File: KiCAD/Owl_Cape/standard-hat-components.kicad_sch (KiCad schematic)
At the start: 12 parts, among them Q1 MMDT5401, Q2 DMG2302U, U1 AT24C256C

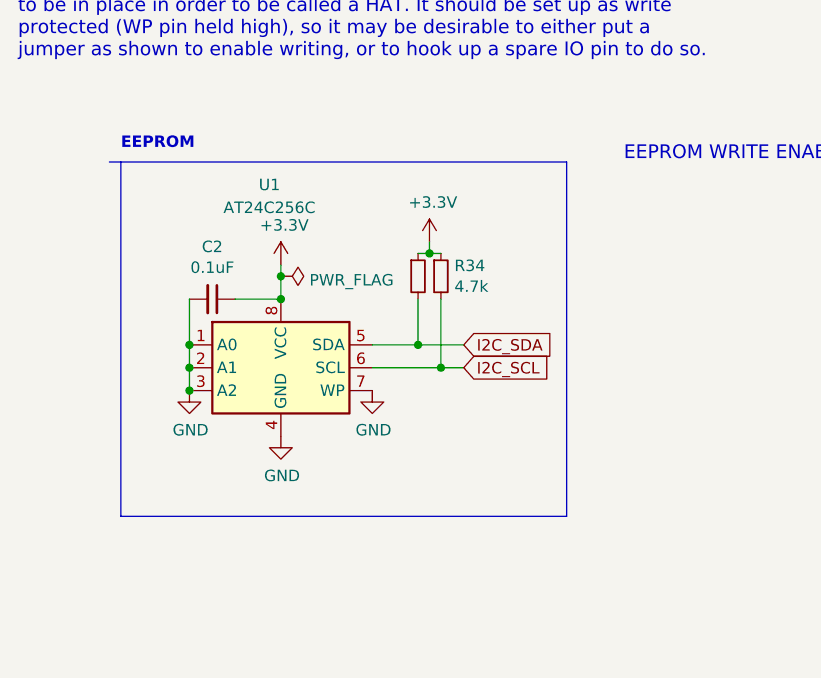
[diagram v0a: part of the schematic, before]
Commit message: formatting fix
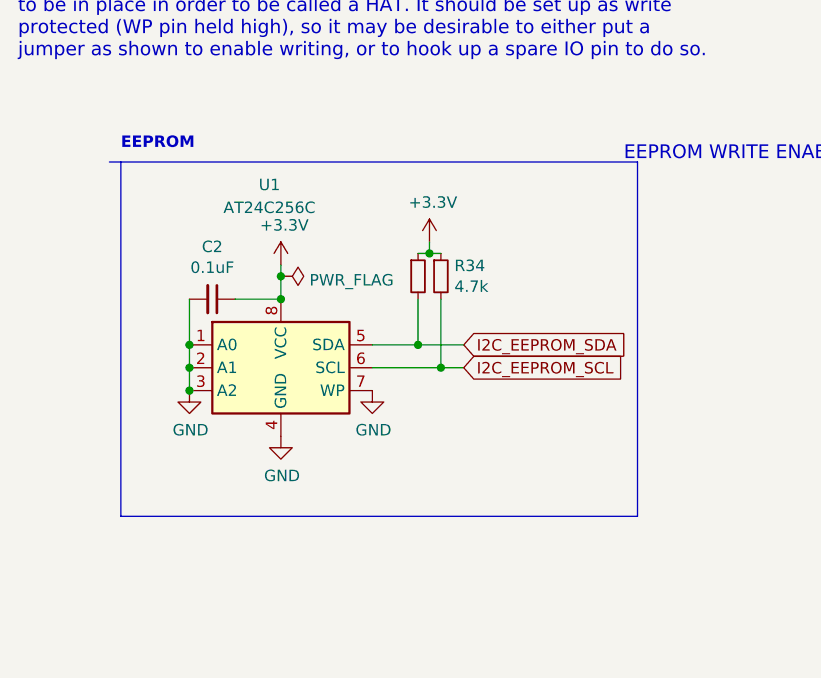
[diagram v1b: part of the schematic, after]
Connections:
- net I2C_SCL renamed I2C_EEPROM_SCL
- net I2C_SDA renamed I2C_EEPROM_SDA
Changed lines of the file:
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@@
     (stroke (width 0) (type default) (color 0 0 0 0))
   )
-  (polyline (pts (xy 80.01 62.23) (xy 80.01 101.6))
+  (polyline (pts (xy 87.884 62.23) (xy 87.884 101.6))
     (stroke (width 0) (type default) (color 0 0 0 0))
   )
@@
     (stroke (width 0) (type default) (color 0 0 0 0))
   )
-  (polyline (pts (xy 80.01 101.6) (xy 30.48 101.6))
+  (polyline (pts (xy 87.884 101.6) (xy 30.48 101.6))
     (stroke (width 0) (type default) (color 0 0 0 0))
   )
@@
     (stroke (width 0) (type default) (color 0 0 0 0))
   )
-  (polyline (pts (xy 29.21 62.23) (xy 80.01 62.23))
+  (polyline (pts (xy 29.21 62.23) (xy 87.884 62.23))
     (stroke (width 0) (type default) (color 0 0 0 0))
   )
@@
     (effects (font (size 1.524 1.524)) (justify left bottom))
   )
-  (global_label "I2C_SCL" (shape input) (at 68.58 85.09 0) (fields_autoplaced)
+  (global_label "I2C_EEPROM_SCL" (shape input) (at 68.58 85.09 0) (fields_autoplaced)
     (effects (font (size 1.27 1.27)) (justify left))
-    (property "Intersheet References" "${INTERSHEET_REFS}" (id 0) (at 3.81 8.89 0)
-      (effects (font (size 1.27 1.27)) hide)
+    (property "Intersheet References" "${INTERSHEET_REFS}" (id 0) (at 87.0513 85.0106 0)
+      (effects (font (size 1.27 1.27)) (justify left) hide)
     )
   )
-  (global_label "I2C_SDA" (shape input) (at 68.58 82.55 0) (fields_autoplaced)
+  (global_label "I2C_EEPROM_SDA" (shape input) (at 68.58 82.55 0) (fields_autoplaced)
     (effects (font (size 1.27 1.27)) (justify left))
-    (property "Intersheet References" "${INTERSHEET_REFS}" (id 0) (at 3.81 8.89 0)
-      (effects (font (size 1.27 1.27)) hide)
+    (property "Intersheet References" "${INTERSHEET_REFS}" (id 0) (at 87.1118 82.4706 0)
+      (effects (font (size 1.27 1.27)) (justify left) hide)
     )
   )
